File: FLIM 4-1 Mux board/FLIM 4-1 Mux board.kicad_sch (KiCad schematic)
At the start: 23 parts, among them J1 Conn_01x14_Pin, J2 Conn_01x14_Pin, J3 Conn_01x05_Pin, SW1 SW_Push_LED, U1 PTMUX8109PWR, U2 DI79L18UAB, U3 DI78L18UAB, U4 Itsy_Bitsy_32u4

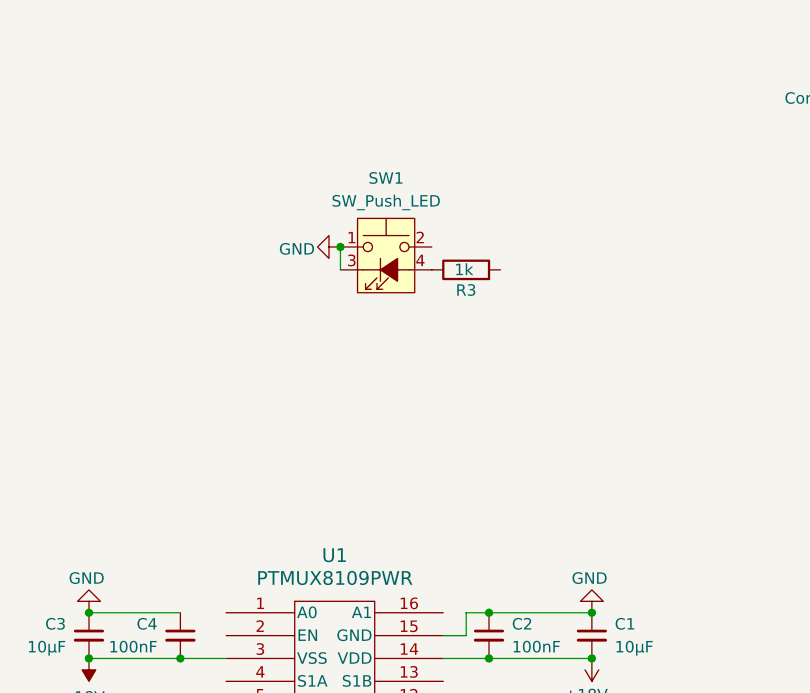
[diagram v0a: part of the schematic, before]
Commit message: Last update before change to cascade RF switches
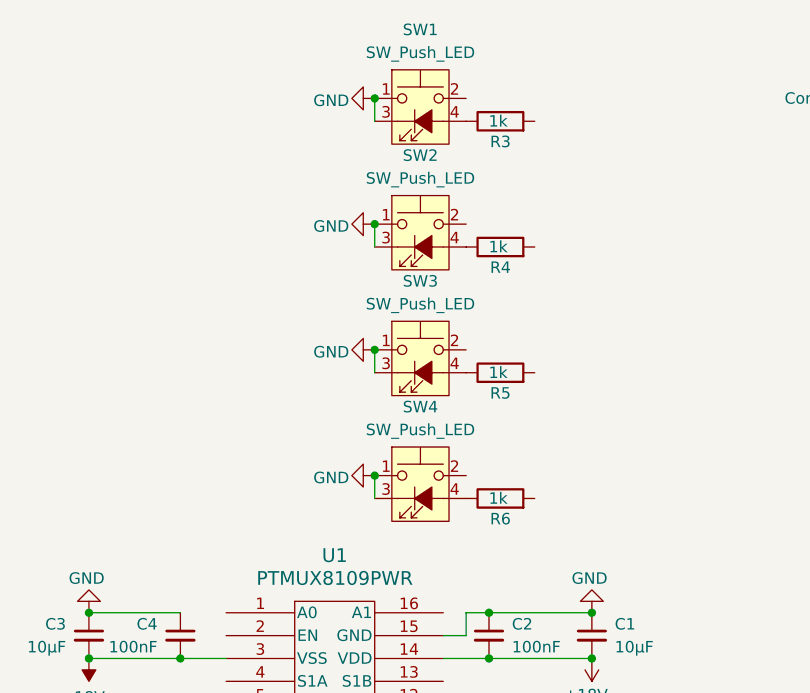
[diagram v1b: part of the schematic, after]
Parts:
- added R4, R5, R6: 1k, Resistor_SMD:R_0805_2012Metric, symbol Device:R
- added SW2, SW3, SW4: SW_Push_LED, Custom:TSSLE 6868 R RNN J, symbol Switch:SW_Push_LED
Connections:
- net GND: now also SW2.1, SW2.3 (K), SW3.1, SW3.3 (K), SW4.1, SW4.3 (K)
- new net: R4.1, SW2.4 (A)
- new net: R5.1, SW3.4 (A)
- new net: R6.1, SW4.4 (A)
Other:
- moved on the sheet: R3, SW1

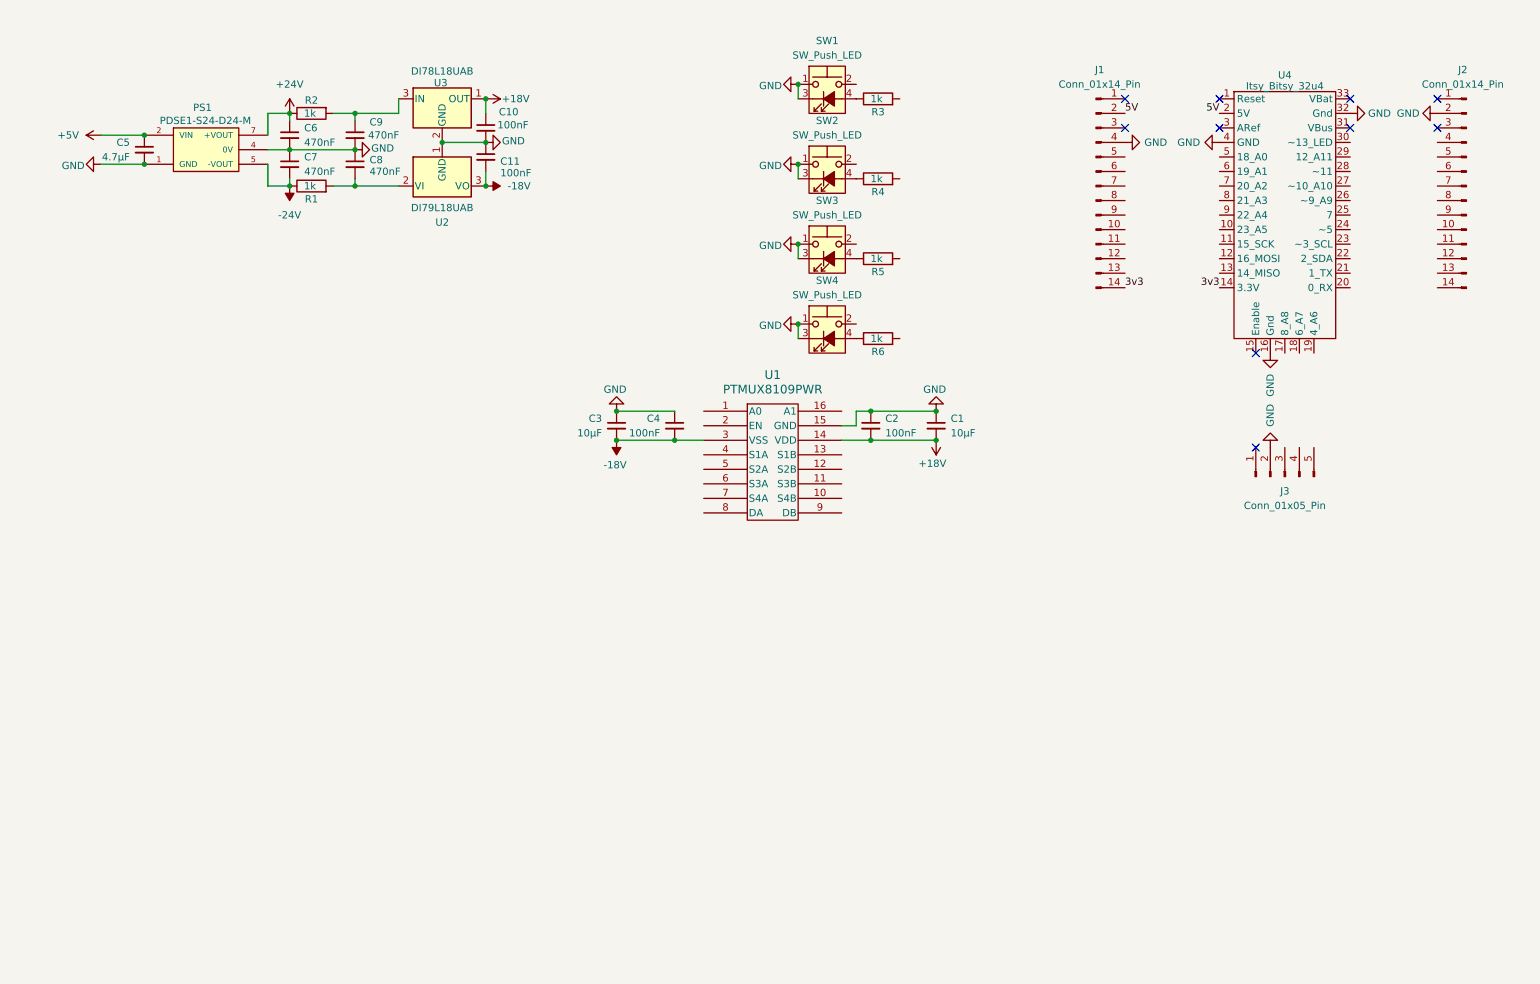
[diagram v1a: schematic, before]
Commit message: Working draft of full setup
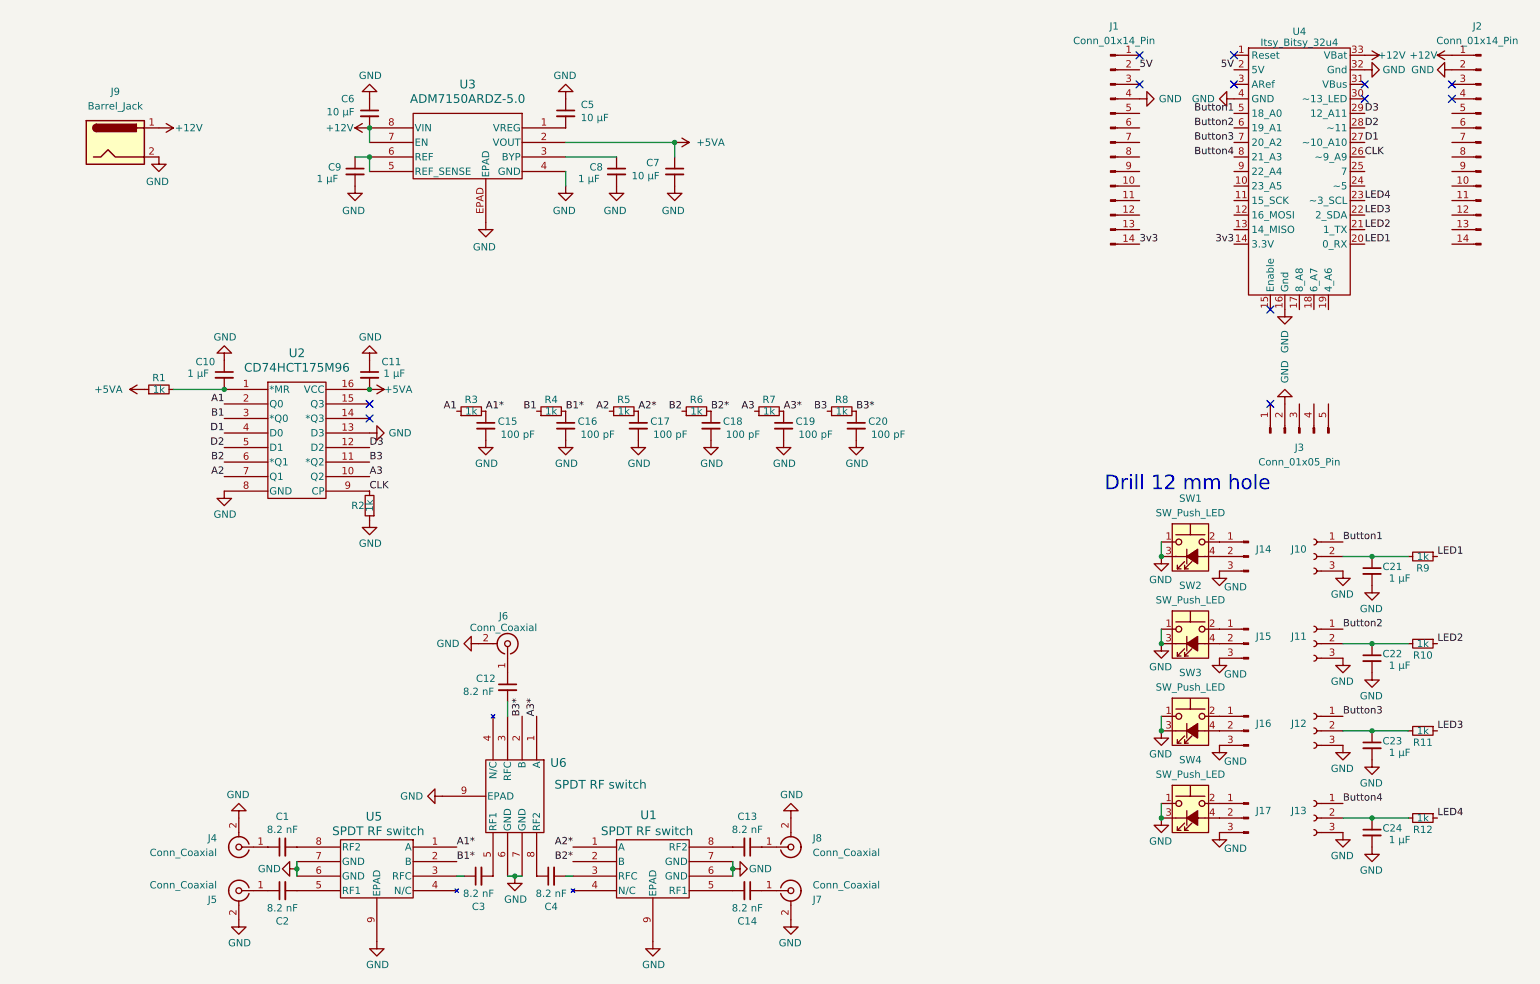
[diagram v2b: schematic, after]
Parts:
- removed PS1: PDSE1-S24-D24-M, PDSE1-S24-D24-M:CONV_PDSE1-S24-D24-M, symbol Custom:PDSE1-S24-D24-M
- removed R1, R2, R3, R4, R5, R6: 1k, Resistor_SMD:R_0805_2012Metric, symbol Device:R
- removed U1: PTMUX8109PWR, TSSOP_8109PWR_TEX, symbol Custom:PTMUX8109PWR
- removed U2: DI79L18UAB, Package_TO_SOT_SMD:SOT-89-3, symbol Regulator_Linear:MCP1703Ax-150xxMB
- removed U3: DI78L18UAB, Package_TO_SOT_SMD:SOT-89-3, symbol Regulator_Linear:MCP1804x-1802xDB
- added C12, C13, C14: 8.2 nF, Capacitor_SMD:C_0402_1005Metric, symbol Device:C_Small
- added C15, C16, C17, C18, C19, C20: 100 pF, Capacitor_SMD:C_0603_1608Metric, symbol Device:C_Small
- added C21, C22, C23, C24: 1 µF, Capacitor_SMD:C_0603_1608Metric, symbol Device:C_Small
- added J10, J11, J12, J13: Conn_01x03_Socket, Connector_PinSocket_2.54mm:PinSocket_1x03_P2.54mm_Vertical_SMD_Pin1Left, symbol Connector:Conn_01x03_Socket
- added J14, J15, J16, J17: Conn_01x03_Pin, symbol Connector:Conn_01x03_Pin
- added J4, J5, J6, J7, J8: Conn_Coaxial, Custom:60312242114510, symbol Connector:Conn_Coaxial
- added J9: Barrel_Jack, Custom:CONN4_00165_TEN, symbol Connector:Barrel_Jack
- added R1, R10, R11, R12, R2, R3, R4, R5, R6, R7, R8, R9: 1k, Resistor_SMD:R_0603_1608Metric, symbol Device:R_Small
- added U1, U5, U6: SPDT RF switch, Custom:MSOP8G_8_ADI, symbol Custom:HMC284AMS8GETR
- added U2: CD74HCT175M96, Custom:74HCT175, symbol Custom:CD74HCT175M96
- added U3: ADM7150ARDZ-5.0, Custom:ADM7150ARDZ-5, symbol Custom:ADM7150ARDZ-5.0
- C1, C3: value 10µF -> 8.2 nF; footprint Capacitor_SMD:C_0805_2012Metric -> Capacitor_SMD:C_0402_1005Metric; Manufacturer Cal-Chip Electronics, Inc. -> Murata Electronics; Part # GMC21X5R106K50NT -> GRM1555C1H822GE01D
- C10, C11: value 100nF -> 1 µF; footprint Capacitor_SMD:C_0805_2012Metric -> Capacitor_SMD:C_0603_1608Metric; Manufacturer Cal-Chip Electronics, Inc. -> Walsin Technology Corporation; Part # GMC21X7R104M100NT -> 0603B105K250CT
- C2, C4: value 100nF -> 8.2 nF; footprint Capacitor_SMD:C_0805_2012Metric -> Capacitor_SMD:C_0402_1005Metric; Manufacturer Cal-Chip Electronics, Inc. -> Murata Electronics; Part # GMC21X7R104M100NT -> GRM1555C1H822GE01D
- C5: value 4.7µF -> 10 µF; footprint Capacitor_SMD:C_0805_2012Metric -> Capacitor_SMD:C_1210_3225Metric; Manufacturer Murata Electronics -> Walsin Technology Corporation; Part # GRM21BR71C475KE51L -> 1210B106M500CT
- C6, C7: value 470nF -> 10 µF; footprint Capacitor_SMD:C_0805_2012Metric -> Capacitor_SMD:C_1210_3225Metric; Manufacturer Samsung Electro-Mechanics -> Walsin Technology Corporation; Part # CL21B474KBFNNNG -> 1210B106M500CT
- C8, C9: value 470nF -> 1 µF; footprint Capacitor_SMD:C_0805_2012Metric -> Capacitor_SMD:C_0603_1608Metric; Manufacturer Samsung Electro-Mechanics -> Walsin Technology Corporation; Part # CL21B474KBFNNNG -> 0603B105K250CT
- SW1, SW2, SW3, SW4: footprint Custom:TSSLE 6868 R RNN J -> (none); Manufacturer Knitter-Switch -> Same Sky (Formerly CUI Devices); Part # TSSLE 6868 R RNN J -> PB4L-M-RR-D-67
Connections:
- net +24V is gone; now on net GND: C6.1
- net +5V is gone; now on net GND: C5.1
- net -24V is gone; now on net GND: C7.2
- net GND: now also C10.1, C8.2, C15.2, C16.2, C17.2, C18.2, C19.2, C20.2, C21.2, C22.2, C23.2, C24.2, J10.3 (Pin_3), J11.3 (Pin_3), J12.3 (Pin_3), J13.3 (Pin_3), J14.3 (Pin_3), J15.3 (Pin_3), J16.3 (Pin_3), J17.3 (Pin_3), J4.2 (Ext), J5.2 (Ext), J6.2 (Ext), J7.2 (Ext), J8.2 (Ext), J9.2, R2.1, U1.6 (GND), U1.7 (GND), U1.9 (EPAD), U2.13 (D3), U2.8 (GND), U3.4 (GND), U3.EPAD, U5.6 (GND), U5.7 (GND), U5.9 (EPAD), U6.6 (GND), U6.7 (GND), U6.9 (EPAD); no longer C1.1, C10.2, C2.1, C3.1, C4.1, C5.2, C6.2, C7.1, C8.1
- net at SW1.2: now also J14.1 (Pin_1)
- net at SW1.4 (A): now also J14.2 (Pin_2)
- net at SW2.4 (A): now also J15.2 (Pin_2)
- net at SW3.4 (A): now also J16.2 (Pin_2)
- net at SW3.2: now also J16.1 (Pin_1)
- net at SW2.2: now also J15.1 (Pin_1)
- net at SW4.4 (A): now also J17.2 (Pin_2)
- net at C9.1: now also U3.5 (REF_SENSE), U3.6 (REF)
- net at SW4.2: now also J17.1 (Pin_1)
- net LED1: now reaches U4.20 (0_RX)
- net LED1: now also R9.1
- net LED2: now reaches U4.21 (1_TX)
- net LED2: now also R10.1
- net LED3: now reaches U4.22 (2_SDA)
- net LED3: now also R11.1
- net LED4: now reaches U4.23 (~3_SCL)
- net LED4: now also R12.1
- net CLK: now reaches U4.26 (~9_A9)
- net CLK: now also R2.2, U2.9 (CP)
- net D1: now reaches U4.27 (~10_A10)
- net D1: now also U2.4 (D0)
- net D2: now reaches U4.28 (~11)
- net D2: now also U2.5 (D1)
- net D3: now reaches U4.29 (12_A11)
- net D3: now also U2.12 (D2)
- net +12V: now reaches U4.33 (VBat)
- net +12V: now also C6.2, J2.1 (Pin_1), J9.1, U3.7 (EN), U3.8 (VIN)
- net Button1: now reaches U4.5 (18_A0)
- net Button1: now also J10.1 (Pin_1)
- net Button2: now reaches U4.6 (19_A1)
- net Button2: now also J11.1 (Pin_1)
- net Button3: now reaches U4.7 (20_A2)
- net Button3: now also J12.1 (Pin_1)
- net Button4: now reaches U4.8 (21_A3)
- net Button4: now also J13.1 (Pin_1)
- removed net +18V: C1.2, C10.1, C2.2
- removed net -18V: C11.2, C3.2, C4.2
- new net: C24.1, J13.2 (Pin_2), R12.2
- new net: C21.1, J10.2 (Pin_2), R9.2
- new net: C22.1, J11.2 (Pin_2), R10.2
- new net: C8.1, U3.3 (BYP)
- new net: C13.1, J8.1 (In)
- new net: C13.2, U1.8 (RF2)
- new net: C5.2, U3.1 (VREG)
- new net: C10.2, R1.2, U2.1 (*MR)
- new net: C12.1, J6.1 (In)
- new net: C23.1, J12.2 (Pin_2), R11.2
- new net: C12.2, U6.3 (RFC)
- new net: C1.1, J4.1 (In)
- new net: C1.2, U5.8 (RF2)
- new net: C3.2, U6.5 (RF1)
- new net: C4.1, U6.8 (RF2)
- new net: C2.1, J5.1 (In)
- new net: C2.2, U5.5 (RF1)
- new net: C4.2, U1.3 (RFC)
- new net: C14.2, U1.5 (RF1)
- new net: C14.1, J7.1 (In)
- new net: C3.1, U5.3 (RFC)
- new net +5VA: C11.2, C7.1, R1.1, U2.16 (VCC), U3.2 (VOUT)
- new net A1: R3.1, U2.2 (Q0)
- new net A1*: C15.1, R3.2, U5.1 (A)
- new net A2: R5.1, U2.7 (Q1)
- new net A2*: C17.1, R5.2, U1.1 (A)
- new net A3: R7.1, U2.10 (Q2)
- new net A3*: C19.1, R7.2, U6.1 (A)
- new net B1: R4.1, U2.3 (*Q0)
- new net B1*: C16.1, R4.2, U5.2 (B)
- new net B2: R6.1, U2.6 (*Q1)
- new net B2*: C18.1, R6.2, U1.2 (B)
- new net B3: R8.1, U2.11 (*Q2)
- new net B3*: C20.1, R8.2, U6.2 (B)
- no-connect marks 10 -> 12
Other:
- note added: "Drill 12 mm hole"
- moved on the sheet: J1, J2, J3, U4

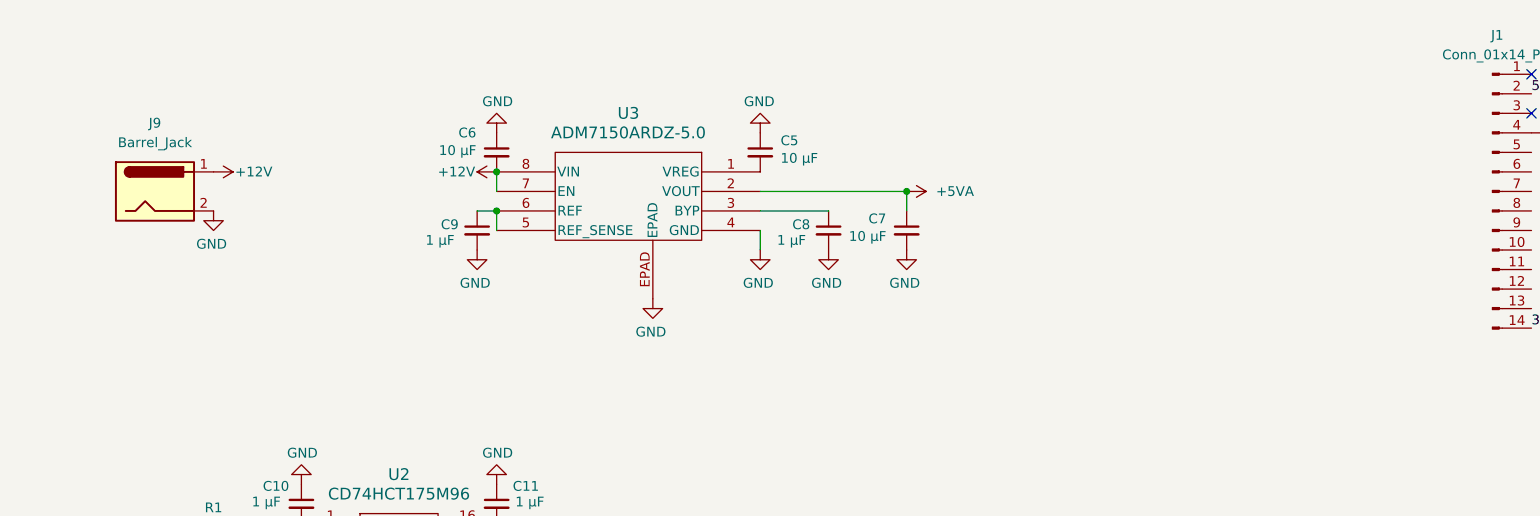
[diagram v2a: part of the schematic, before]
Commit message: non islated DC jack with filter
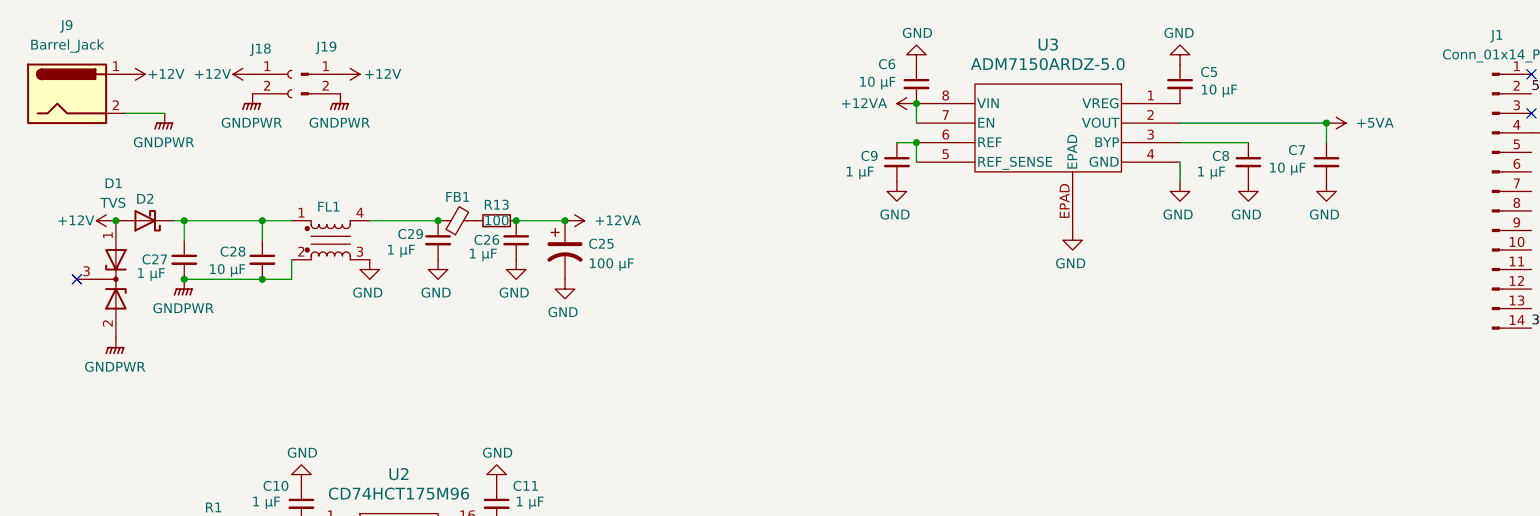
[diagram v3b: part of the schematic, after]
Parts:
- added C25: 100 µF, Capacitor_SMD:CP_Elec_10x10, symbol Device:C_Polarized_US
- added C26, C27, C29: 1 µF, Capacitor_SMD:C_0603_1608Metric, symbol Device:C_Small
- added C28: 10 µF, Capacitor_SMD:C_1210_3225Metric, symbol Device:C_Small
- added D1: TVS, Package_TO_SOT_SMD:SOT-23, symbol Device:D_Zener_Dual_CommonCathode_AAK
- added D2: D_Schottky, Diode_SMD:D_SOD-323, symbol Device:D_Schottky
- added FB1: FerriteBead_Small, Inductor_SMD:L_0603_1608Metric, symbol Device:FerriteBead_Small
- added FL1: Choke_CommonMode_PulseElectronics_PH9455x105NL, Custom:WE-SL2, symbol Filter:Choke_CommonMode_PulseElectronics_PH9455x105NL
- added J18: Conn_01x02_Socket, `, symbol Connector:Conn_01x02_Socket
- added J19: Conn_01x02_Pin, Custom:SAMTEC_TSM-102-02-L-SH, symbol Connector:Conn_01x02_Pin
- added R13: 100, Resistor_SMD:R_0805_2012Metric, symbol Device:R_Small
- J9: footprint Custom:CONN4_00165_TEN -> `; Manufacturer Tensility International Corp -> Switchcraft Inc.; Part # 54-00165 -> 712AFMS
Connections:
- net +12V: now also D1.1 (A), D2.2 (A), J18.1 (Pin_1), J19.1 (Pin_1); no longer C6.2, U3.7 (EN), U3.8 (VIN)
- net GND: now also C25.2, C26.2, C29.2, FL1.3; no longer J9.2
- new net: C29.1, FB1.1, FL1.4
- new net: C27.1, C28.1, D2.1 (K), FL1.1
- new net: FB1.2, R13.1
- new net +12VA: C25.1, C26.1, C6.2, R13.2, U3.7 (EN), U3.8 (VIN)
- new net GNDPWR: C27.2, C28.2, D1.2 (A), FL1.2, J18.2 (Pin_2), J19.2 (Pin_2), J9.2
- no-connect marks 12 -> 13
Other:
- moved on the sheet: C5, C6, C7, C8, C9, J9, U3
